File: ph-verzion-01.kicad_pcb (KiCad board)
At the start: 2 copper layers, 190 x 120 mm, 104 parts, among them J1 230V_IN, J10 OUT4, J11 AC_OUT_230V, J12 12V_IO, J2 DISPLAY, J3 1W_1, J4 1W_2, J5 1W_3, J6 1W_4, J7 GPIO_EXT, J8 UART, J9 OUT3, P1 pH_BNC, P2 ORP_BNC, Q1 IRLR2905, Q2 IRLR2905, Q3 IRLR2905, Q4 IRLR2905, U1 HLK-30M12, U10 ADS1115, U11 ESP32-WROOM-32E-N4, U12 LTV-356T, U2 LM2596S-5.0, U3 LD1117AS33TR, U4 L7805ABD2T, U5 TPS60400, U6 CA3140EZ, U7 TL071IP, U8 CA3140EZ, U9 TL071IP

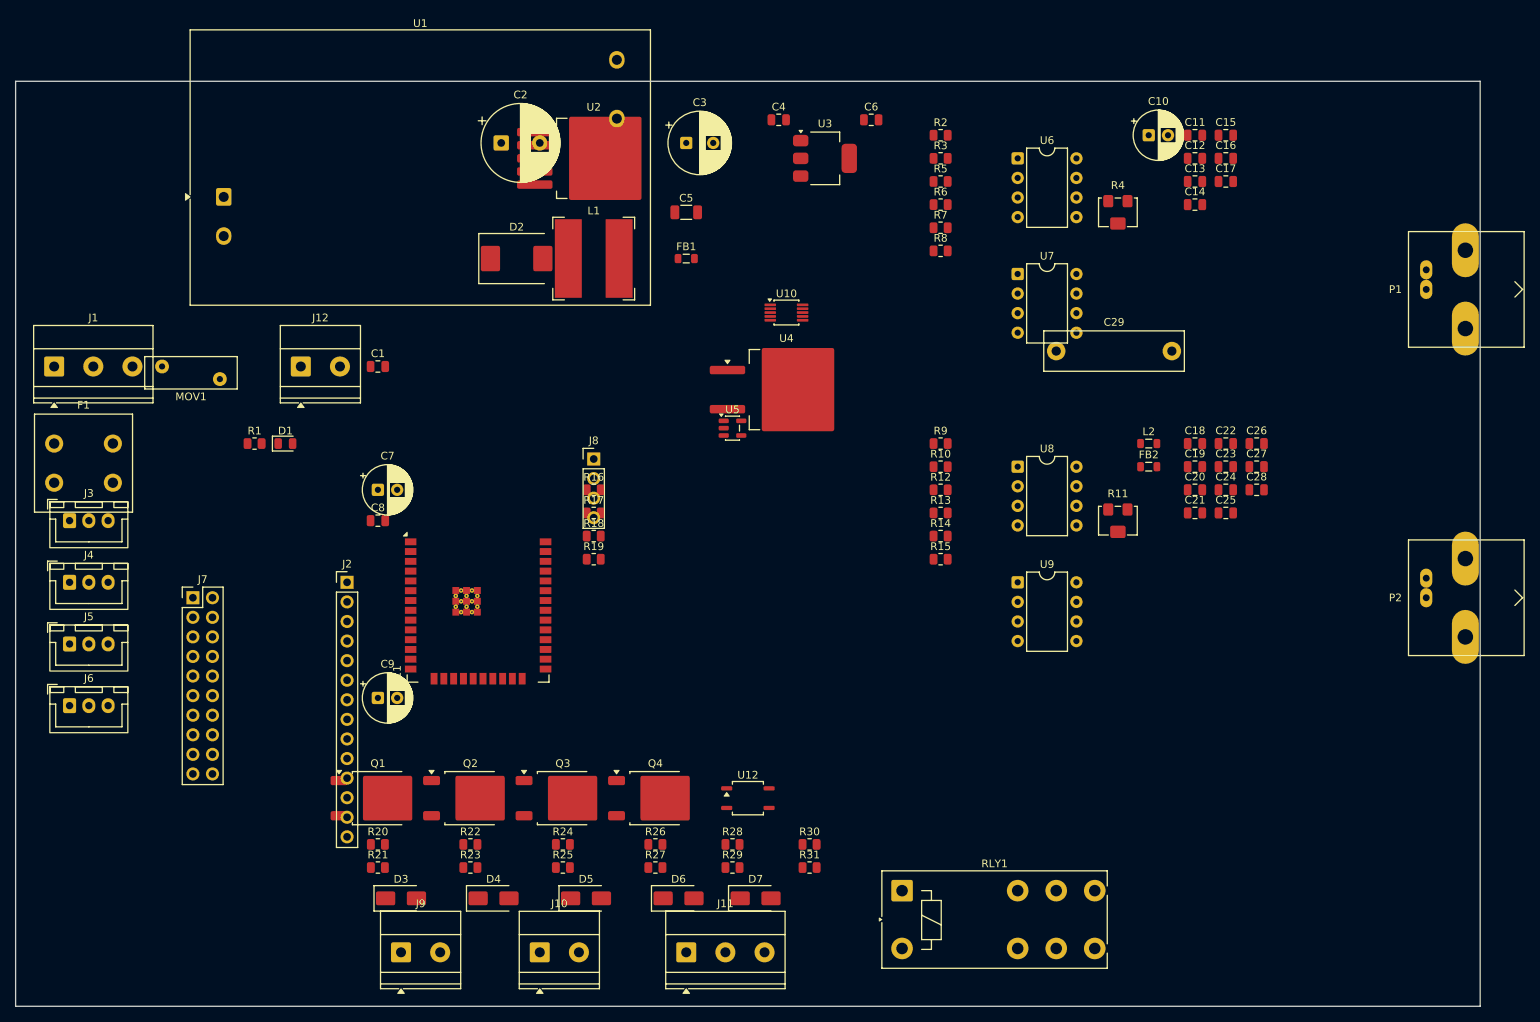
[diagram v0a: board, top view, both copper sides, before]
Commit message: jedit
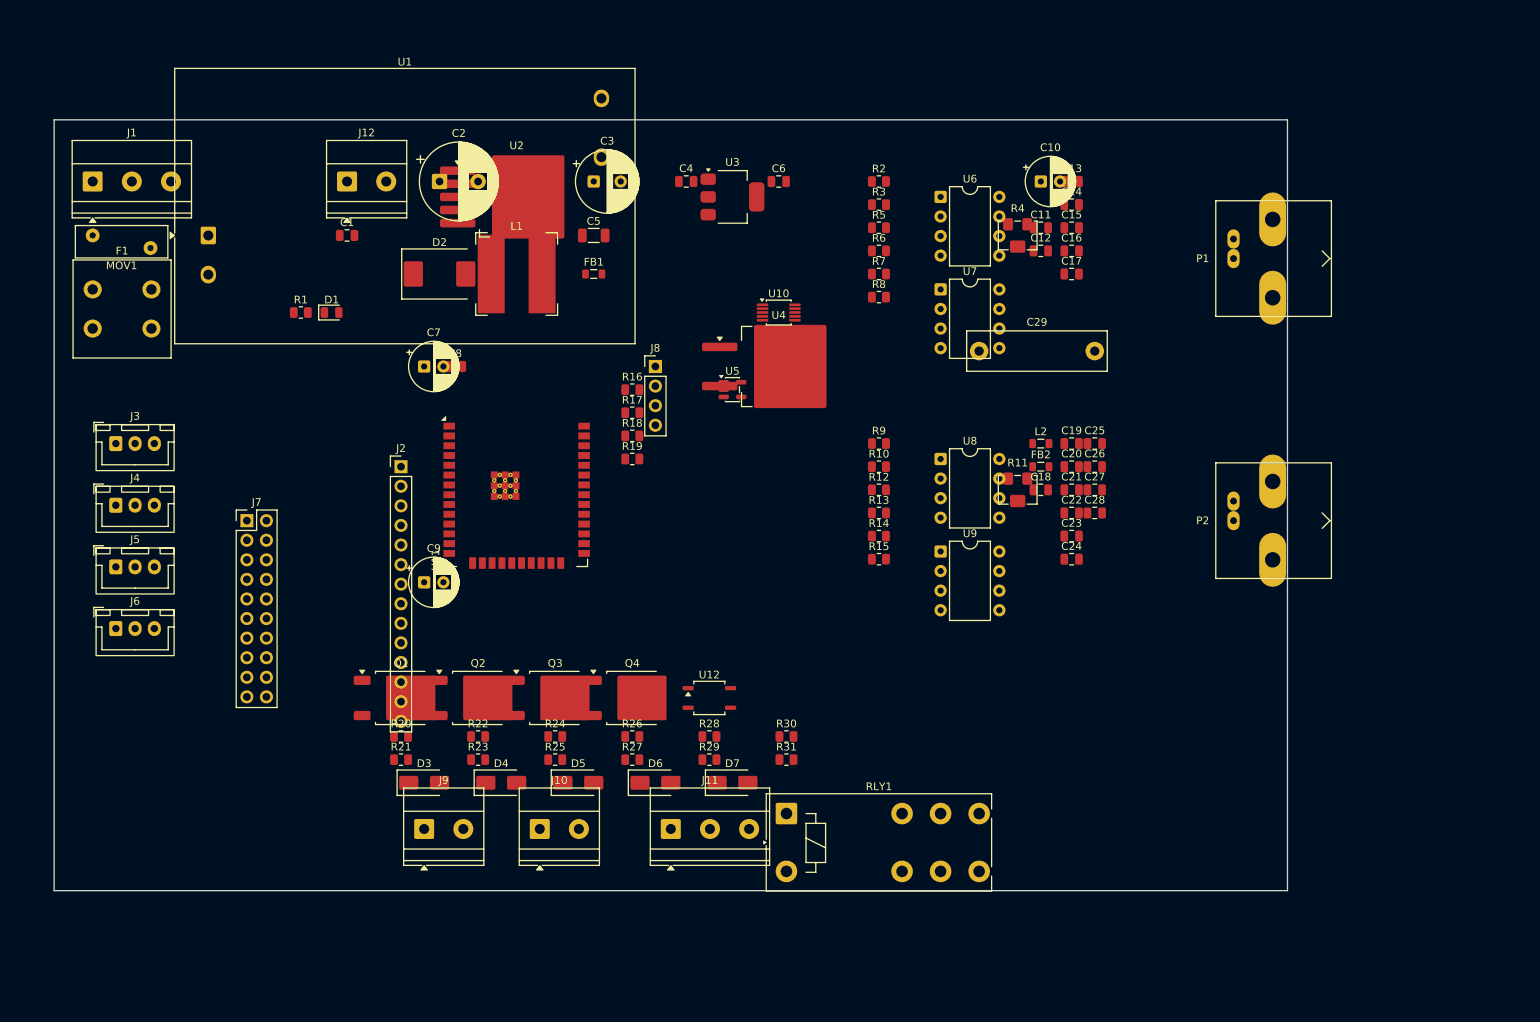
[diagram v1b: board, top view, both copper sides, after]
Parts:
- moved P2 26.9 mm to (183.0, 82.0)
- moved P1 25.3 mm to (183.0, 48.0)
- moved J12 24.7 mm to (68.0, 38.0)
- moved J1 24.5 mm to (35.0, 38.0)
- moved C11 23.3 mm to (158.0, 44.0)
- moved C12 23.3 mm to (158.0, 47.0)
- moved C15 23.3 mm to (162.0, 44.0)
- moved C16 23.3 mm to (162.0, 47.0)
- moved C17 23.3 mm to (162.0, 50.0)
- moved C8 22.4 mm to (82.0, 62.0)
- moved C22 21.9 mm to (162.0, 81.0)
- moved C23 21.9 mm to (162.0, 84.0)
- moved C24 21.9 mm to (162.0, 87.0)
- moved C26 21.2 mm to (165.0, 75.0)
- moved C27 21.2 mm to (165.0, 78.0)
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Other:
- board size 190 x 120 mm -> 160 x 100 mm
